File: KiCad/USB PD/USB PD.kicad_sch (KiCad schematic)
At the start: 38 parts, among them J10 CFG, J11 SEL, J12 Conn_01x03_Pin, J12 GND, J18 Conn_01x02_Pin, J7 VCC, J8 ESP32 Jumpers, J8 TX, J9 RX, U1 AO3400A, U2 IP2721, U4 TYPE-C_6P, U5 TPS5430DDAR

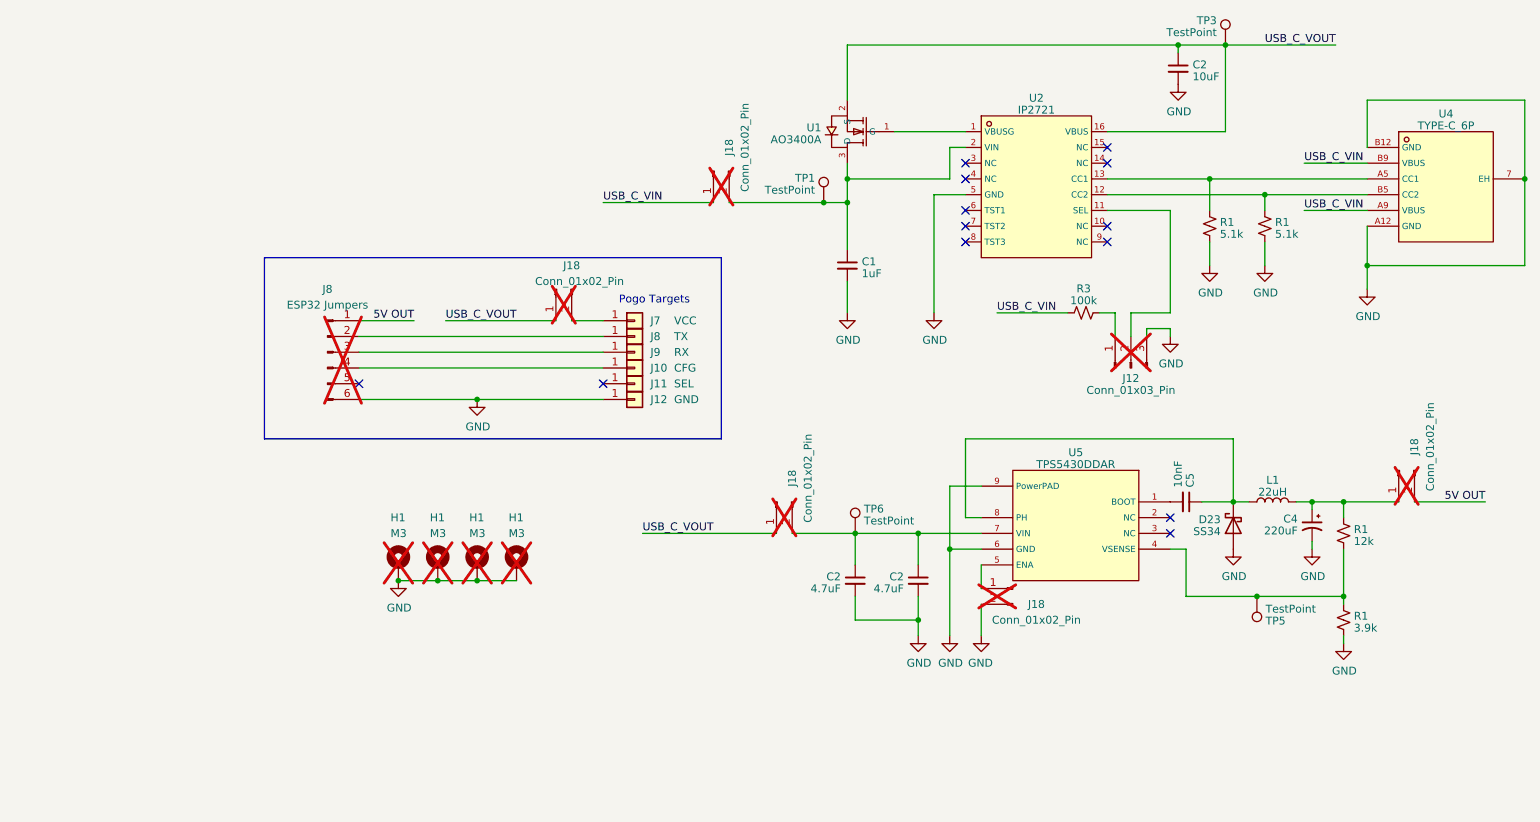
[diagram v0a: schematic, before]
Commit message: Final Commit for 4022S
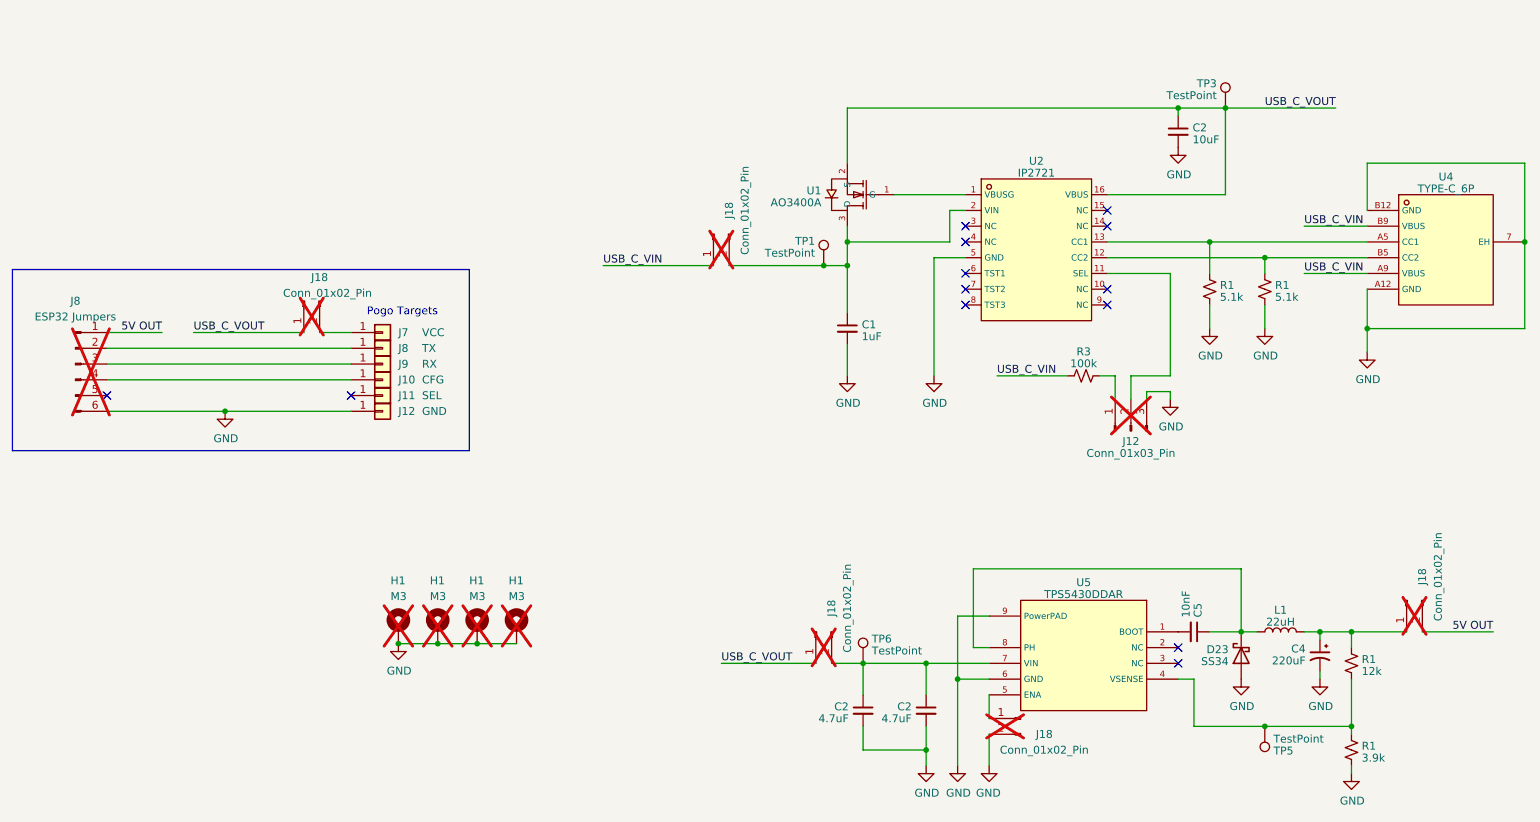
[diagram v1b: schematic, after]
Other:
- moved on the sheet: C1, C2, C4, C5, D23, H1, J10, J11, J12, J18, J7, J8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
